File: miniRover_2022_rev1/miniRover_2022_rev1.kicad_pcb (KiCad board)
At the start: 2 copper layers, 101.6 x 121.9 mm, 15 parts, among them J1 XT60-M, U1 OKI, U2 DRV8871-Breakout-PCB, U3 DRV8871-Breakout-PCB, U4 DRV8871-Breakout-PCB, U5 DRV8871-Breakout-PCB, U6 DRV8871-Breakout-PCB, U7 DRV8871-Breakout-PCB

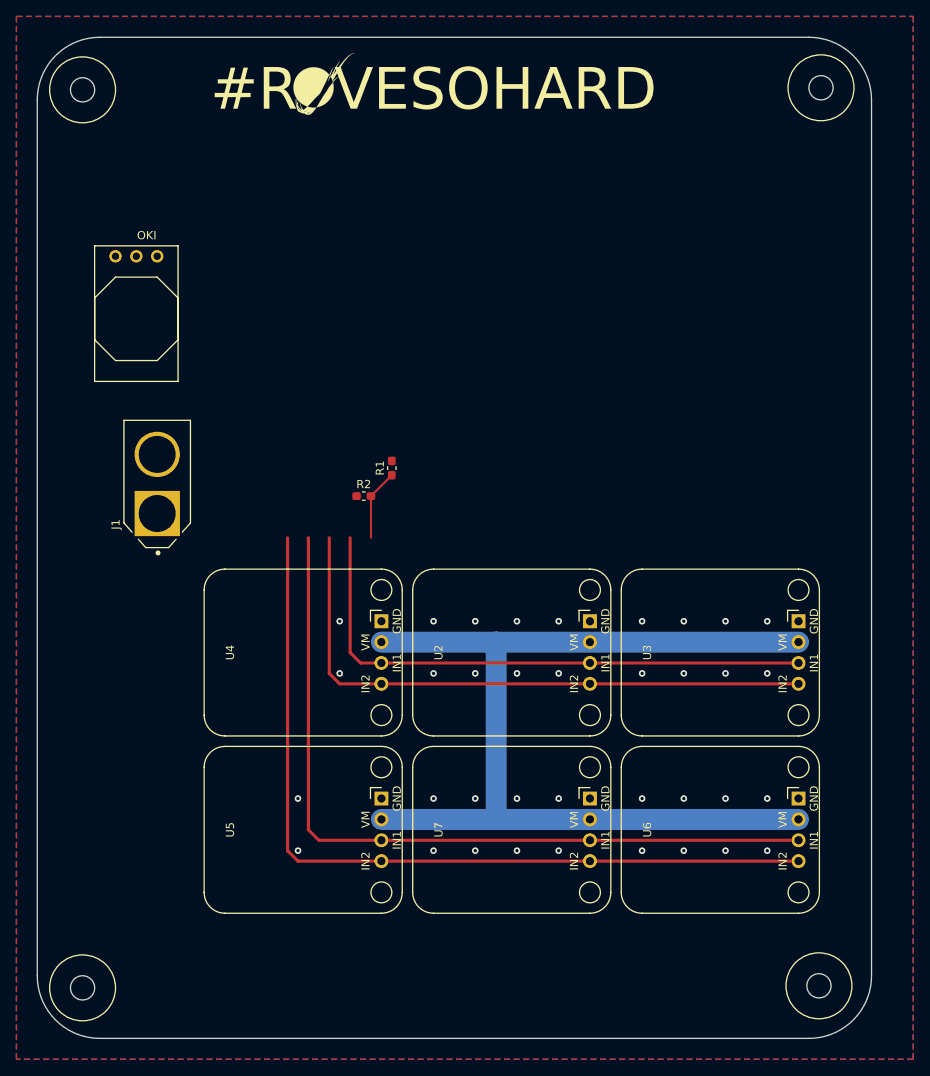
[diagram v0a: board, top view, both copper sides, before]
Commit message: rev1 finished, will be reviewing over the following days
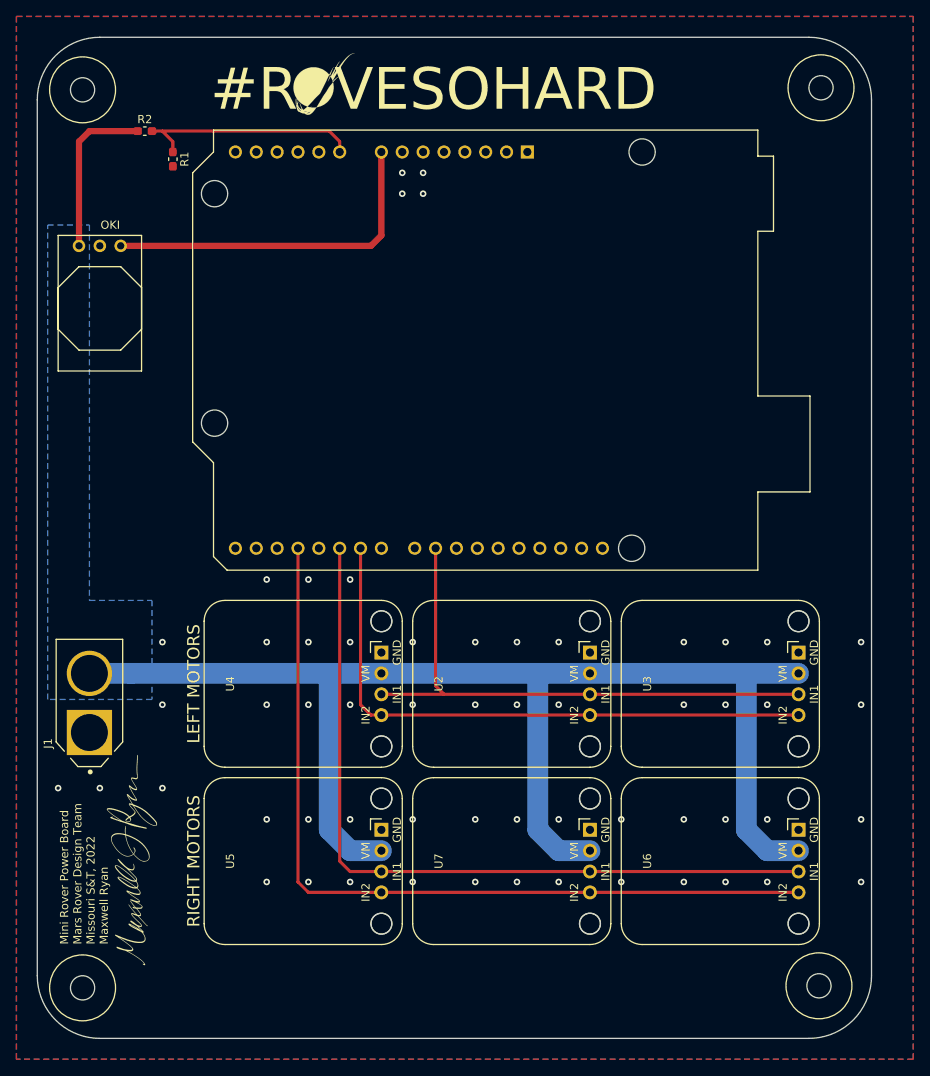
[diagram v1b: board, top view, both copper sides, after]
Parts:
- added A1: Arduino_UNO_R3, Module:Arduino_UNO_R3_WithMountingHoles, B.Cu at (174.0, 29.2)
- added G***: LOGO, MRDT_Silkscreens:0_MRDT_Logo_7.5mm, B.Cu at (176.5, 21.0)
- added G***: LOGO, miniRover2022:maxsignature, F.Cu at (125.7, 115.6)
- moved R2 51.8 mm to (127.4, 26.7)
- moved R1 46.1 mm to (130.8, 30.1), turned to 270 degrees
- moved J1 27.9 mm to (120.7, 96.3)
- moved U1 4.62 mm to (119.4, 40.6)
- moved U2 3.81 mm to (181.6, 90.2)
- moved U3 3.81 mm to (207.0, 90.2)
- moved U4 3.81 mm to (156.2, 90.2)
- moved U5 3.81 mm to (156.2, 111.8)
- moved U6 3.81 mm to (207.0, 111.8)
- moved U7 3.81 mm to (181.6, 111.8)
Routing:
- net +12V: track 123.2 -> 186.1 mm
- net +5V: track 0.00 -> 42.4 mm
- net Net-(A1-Pad9): track 8.67 -> 27.7 mm
- net /motorControllers/RIN1: track 95.8 -> 94.5 mm
- net /motorControllers/RIN2: track 100.9 -> 102.1 mm
- net /motorControllers/LIN2: track 74.2 -> 72.9 mm
- net GND: vias 36 -> 58
- added copper zone on B.Cu, net +12V
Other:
- outline, holes or cut-outs redrawn
- board text added: "LEFT MOTORS"
- board text added: "Mini Rover Power Board Mars Rover Design Team Missouri S&T, 2022 Maxwell Ryan"
- board text added: "RIGHT MOTORS"
